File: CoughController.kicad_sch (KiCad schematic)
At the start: 4 parts, among them J6 電源入力, J7 電源出力

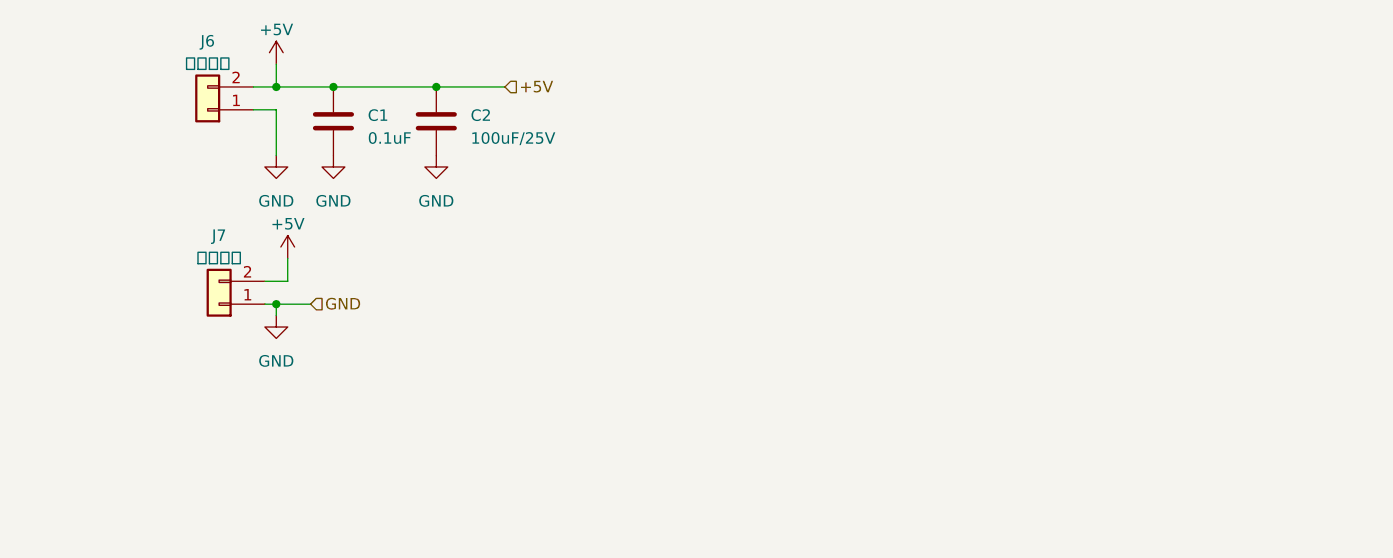
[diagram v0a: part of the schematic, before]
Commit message: カフコントローラ
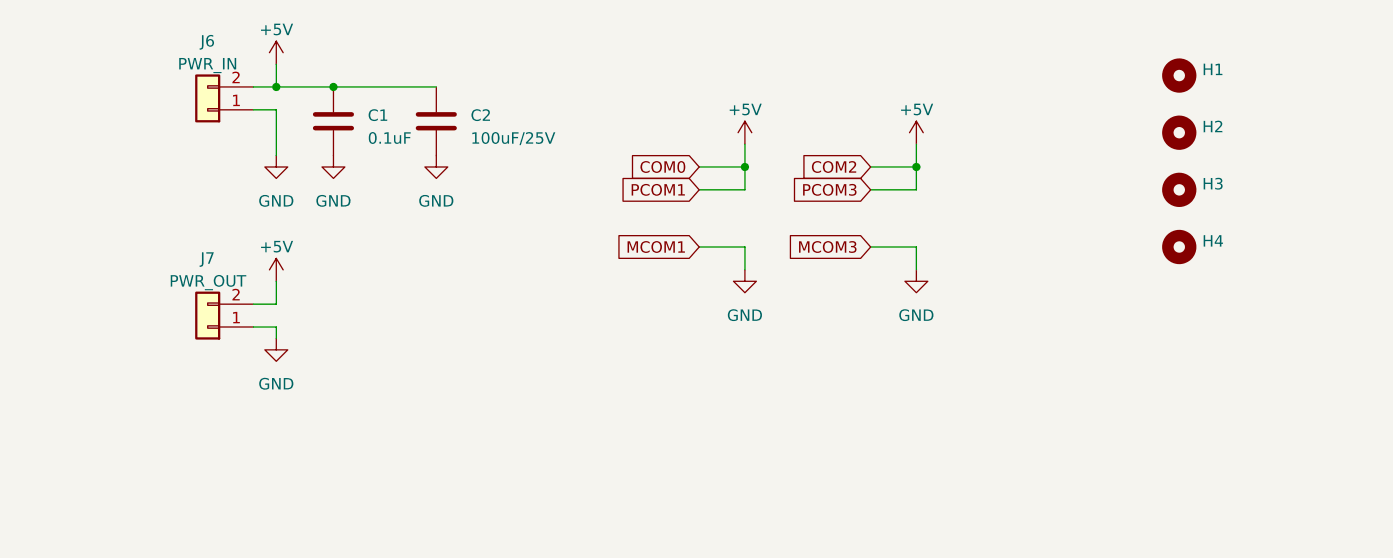
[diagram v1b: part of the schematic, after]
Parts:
- added H1, H2, H3, H4: MountingHole, MountingHole:MountingHole_3.2mm_M3, symbol Mechanical:MountingHole
- J6: value 電源入力 -> PWR_IN
- J7: value 電源出力 -> PWR_OUT
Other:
- moved on the sheet: J7
